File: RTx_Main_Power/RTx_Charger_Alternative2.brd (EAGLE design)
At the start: 102.9 x 43.2 mm, 11 parts, among them IC1 TL331, Q1 STW11NM80

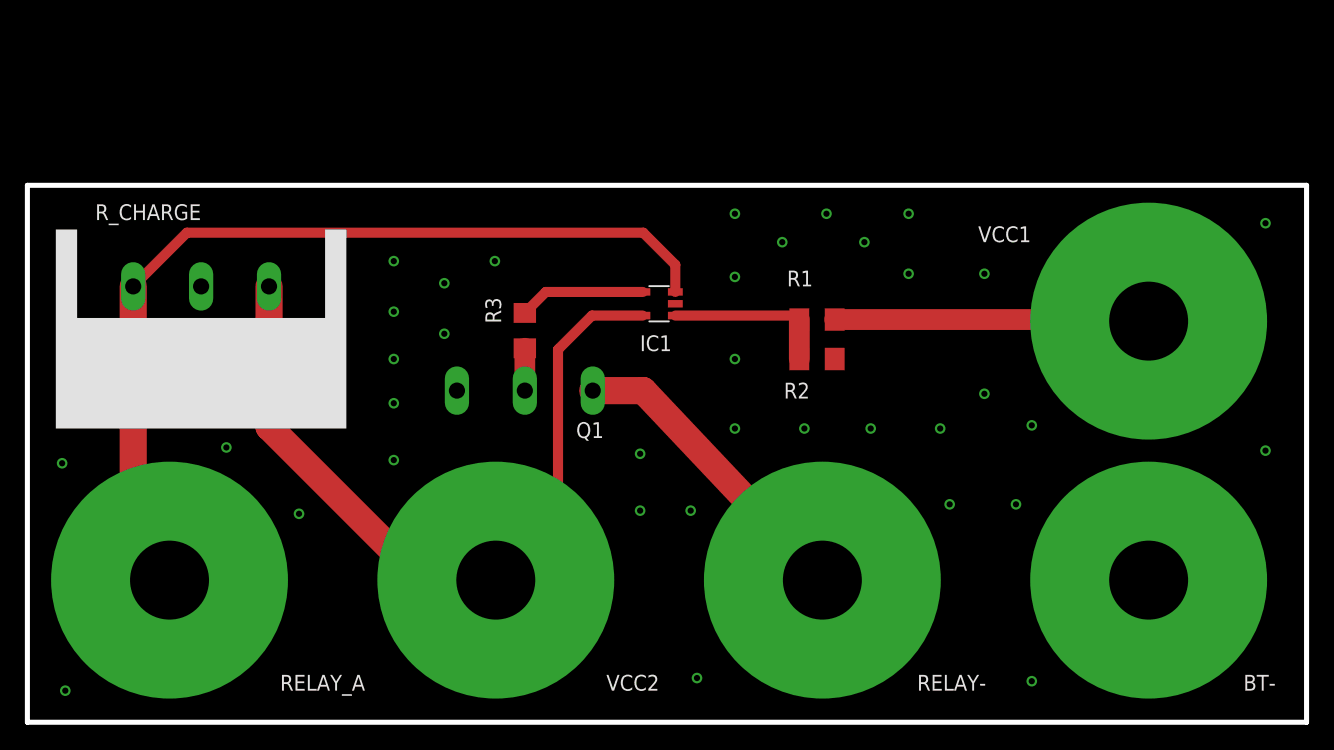
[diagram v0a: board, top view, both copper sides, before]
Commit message: Changes to RTx charger board.
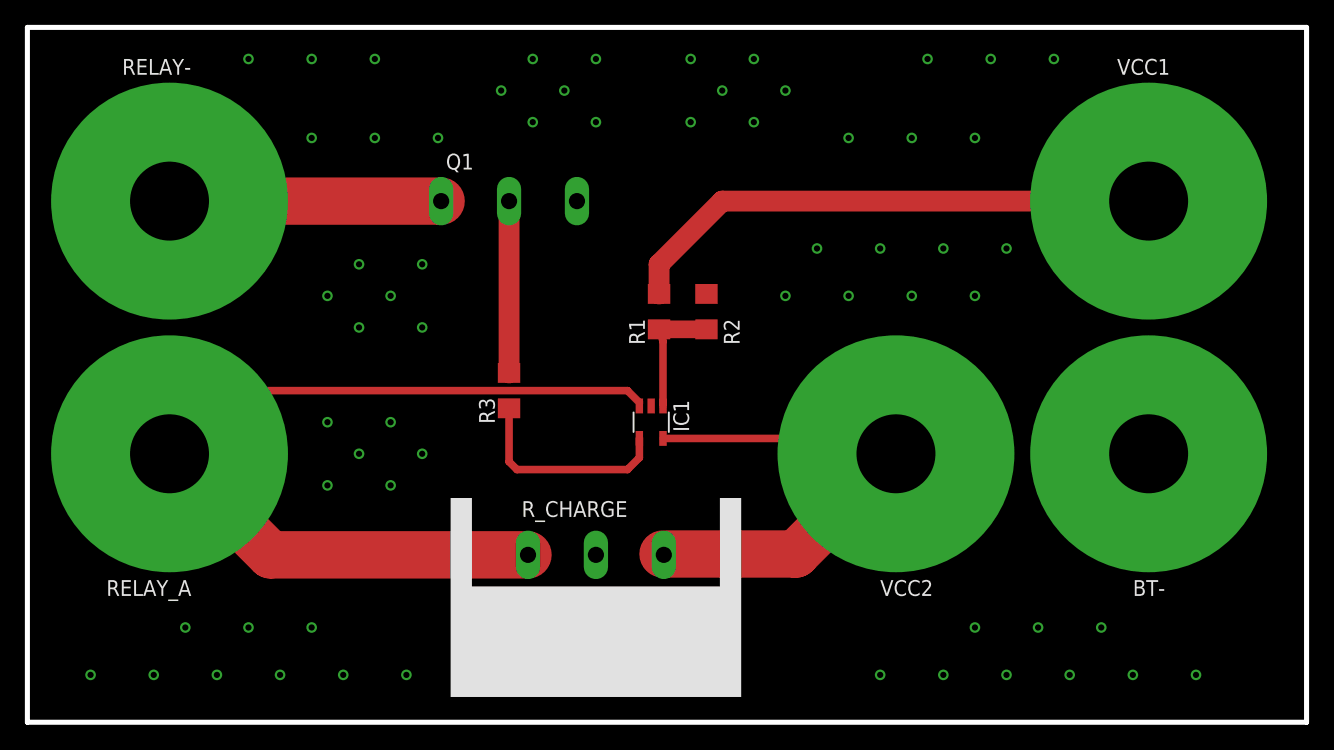
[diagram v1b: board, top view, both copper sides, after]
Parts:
- moved RELAY- 60.7 mm to (11.4, 41.9)
- moved R_CHARGE 38.4 mm to (45.7, 8.89)
- moved VCC2 33.7 mm to (69.8, 21.6)
- moved Q1 15.3 mm to (38.7, 41.9), turned to 0 degrees
- moved R1 12.7 mm to (50.8, 33.0), turned to 90 degrees
- moved BT- 10.2 mm to (90.2, 21.6)
- moved RELAY_A 10.2 mm to (11.4, 21.6)
- moved R2 9.67 mm to (54.6, 33.0), turned to 90 degrees
- moved VCC1 9.65 mm to (90.2, 41.9)
- moved IC1 9.55 mm to (50.2, 24.1), turned to 180 degrees
- moved R3 4.99 mm to (38.7, 26.7), turned to 270 degrees
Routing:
- net VCC2: track 63.3 -> 41.4 mm
- net VCC1: track 25.3 -> 43.9 mm
- net N$5: track 3.40 -> 13.8 mm
- net N$1: track 10.2 -> 17.0 mm
- net REFERENCE: track 13.3 -> 10.0 mm
- net RELAY-: track 25.0 -> 21.8 mm
- net RELAY_A: track 73.5 -> 72.5 mm
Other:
- board size 102.9 x 43.2 mm -> 102.9 x 55.9 mm
